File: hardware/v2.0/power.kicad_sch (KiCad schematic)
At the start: 53 parts, among them U1 ECP5U-25F-CABGA256, U2 LTC3407AEDD-2_PBF, U3 TLV62569DBV

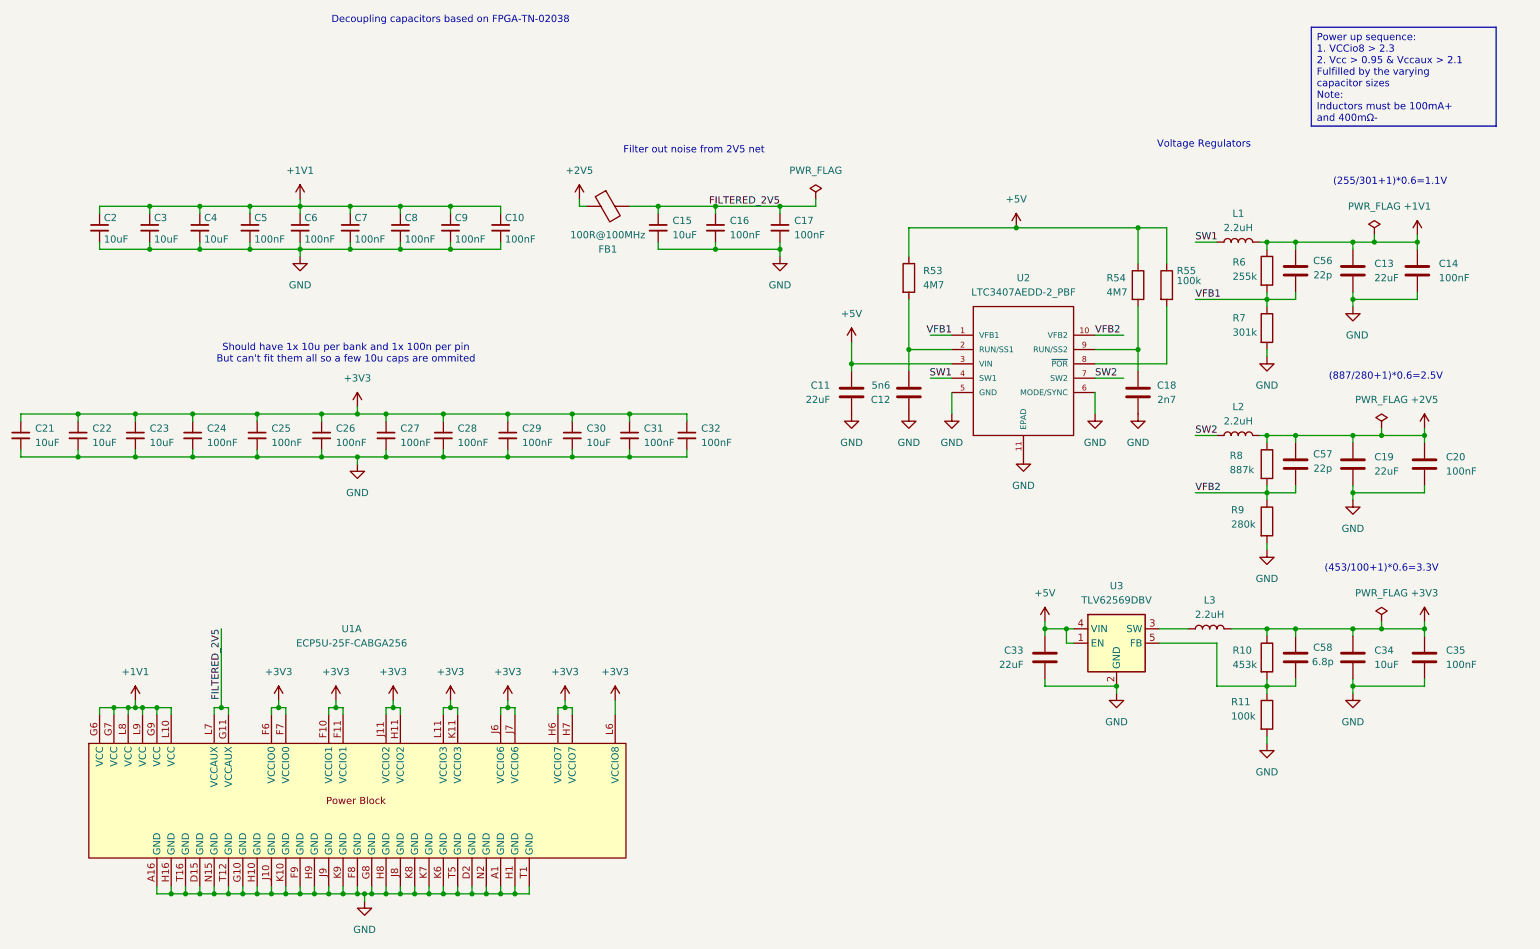
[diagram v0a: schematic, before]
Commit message: ADC power
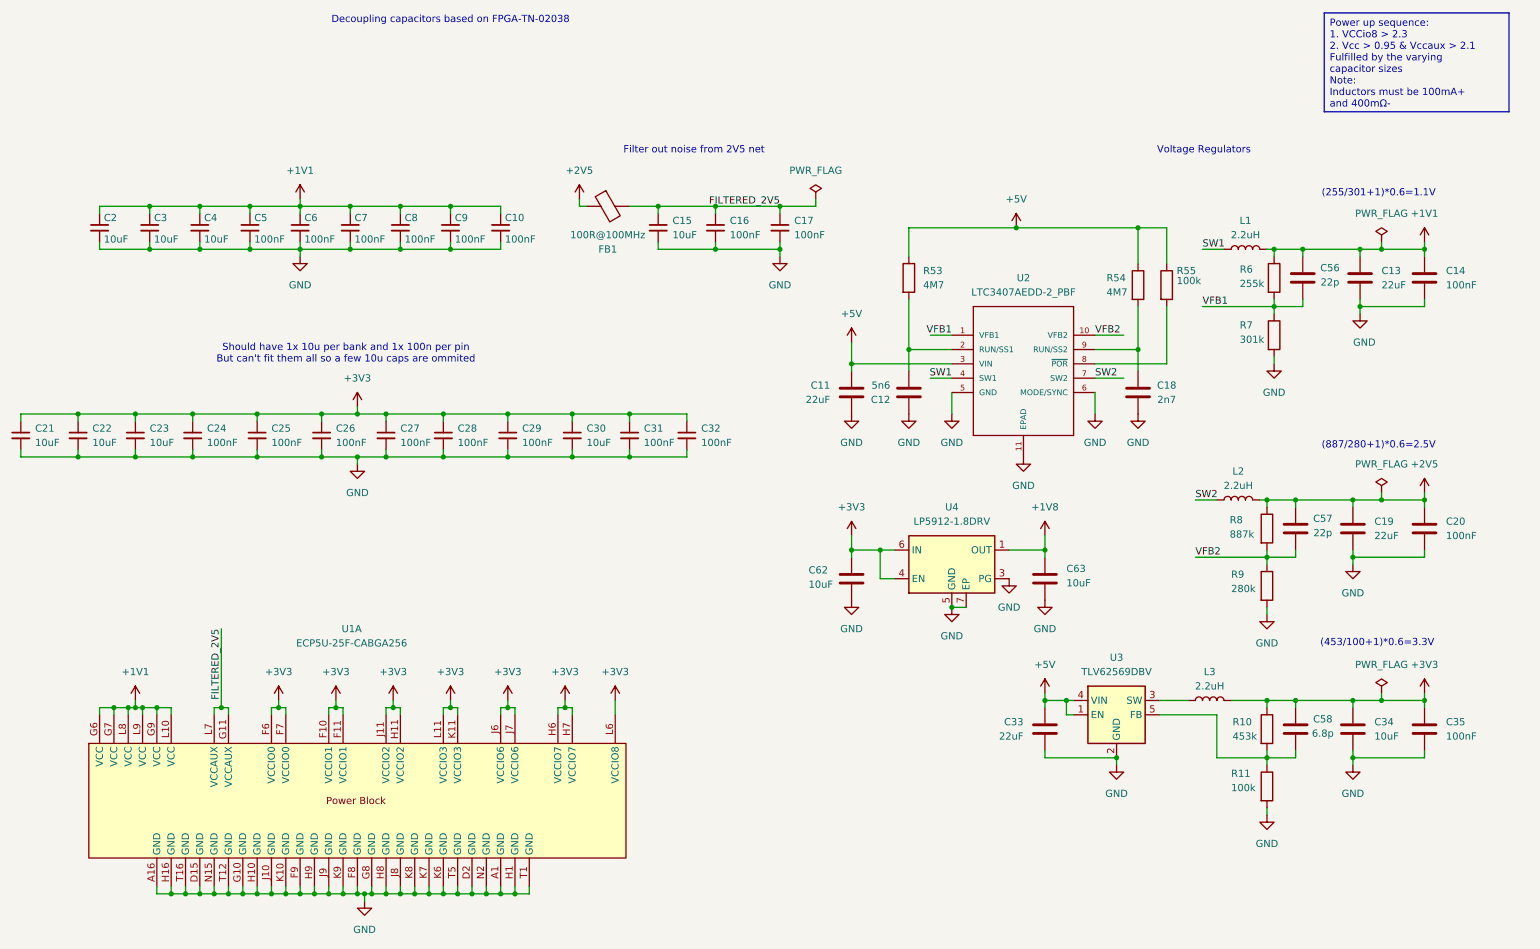
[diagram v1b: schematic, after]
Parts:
- added C62, C63: 10uF, Capacitor_SMD:C_0603_1608Metric, symbol Device:C
- added U4: LP5912-1.8DRV, Package_SON:WSON-6-1EP_2x2mm_P0.65mm_EP1x1.6mm_ThermalVias, symbol Regulator_Linear:LP5912-1.8DRV
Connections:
- net +3V3: now also C62.1, U4.4 (EN), U4.6 (IN)
- net GND: now also C62.2, C63.2, U4.3 (PG), U4.5 (GND), U4.7 (EP)
- new net +1V8: C63.1, U4.1 (OUT)
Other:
- moved on the sheet: C13, C14, C19, C20, C33, C34, C35, C56, C57, C58, L1, L2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
